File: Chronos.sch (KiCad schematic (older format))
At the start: 27 parts, among them Q1 NSS40301MZ4T1G, U1 ATMEGA32U2-AU, Y1 16MHz

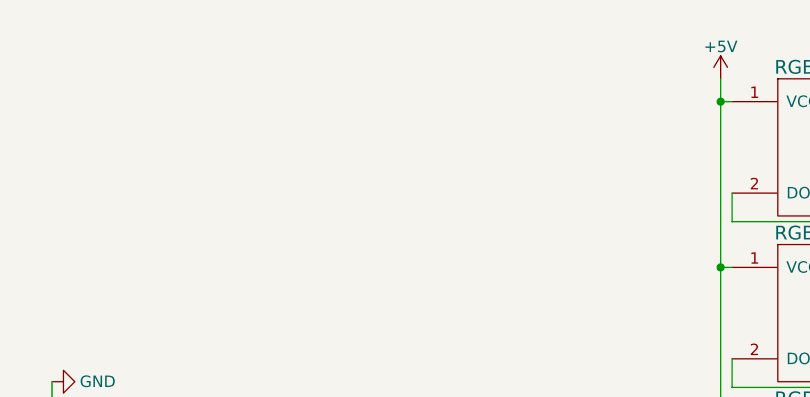
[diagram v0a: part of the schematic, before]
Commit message: Add RGB Decoupling capacitors
Also fix label on matrix sheet being misplaced
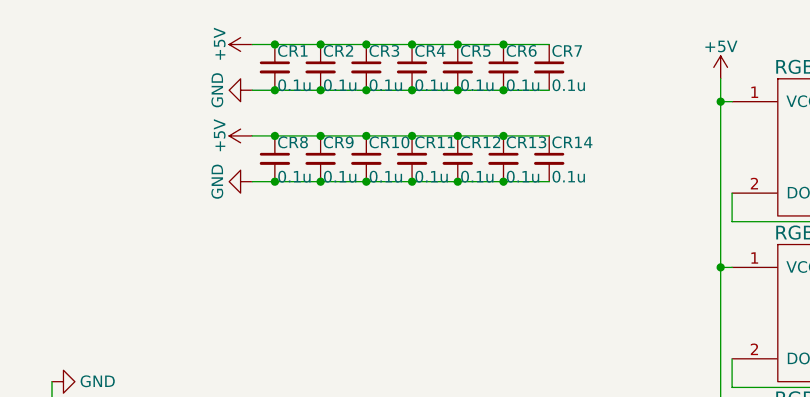
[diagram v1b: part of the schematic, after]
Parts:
- added CR1, CR10, CR11, CR12, CR13, CR14, CR2, CR3, CR4, CR5, CR6, CR7, CR8, CR9: 0.1u, symbol C_Small
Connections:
- net +5V: now also CR1.1, CR10.1, CR11.1, CR12.1, CR13.1, CR14.1, CR2.1, CR3.1, CR4.1, CR5.1, CR6.1, CR7.1, CR8.1, CR9.1
- net GND: now also CR1.2, CR10.2, CR11.2, CR12.2, CR13.2, CR14.2, CR2.2, CR3.2, CR4.2, CR5.2, CR6.2, CR7.2, CR8.2, CR9.2
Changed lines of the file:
@@
 Text Notes 8125 7650 0    60   ~ 0
 2017-10-15\n
+$Comp
+L C_Small CR1
+U 1 1 59E874F1
+P 6450 925
+F 0 "CR1" H 6460 995 50  0000 L CNN
+F 1 "0.1u" H 6460 845 50  0000 L CNN
+F 2 "" H 6450 925 50  0001 C CNN
+F 3 "" H 6450 925 50  0001 C CNN
+	1    6450 925
+	1    0    0    -1
+$EndComp
+$Comp
+L C_Small CR2
+U 1 1 59E879A6
+P 6650 925
+F 0 "CR2" H 6660 995 50  0000 L CNN
+F 1 "0.1u" H 6660 845 50  0000 L CNN
+F 2 "" H 6650 925 50  0001 C CNN
+F 3 "" H 6650 925 50  0001 C CNN
+	1    6650 925
+	1    0    0    -1
+$EndComp
+$Comp
+L C_Small CR3
+U 1 1 59E87A25
+P 6850 925
+F 0 "CR3" H 6860 995 50  0000 L CNN
+F 1 "0.1u" H 6860 845 50  0000 L CNN
+F 2 "" H 6850 925 50  0001 C CNN
+F 3 "" H 6850 925 50  0001 C CNN
+	1    6850 925
+	1    0    0    -1
+$EndComp
+$Comp
+L C_Small CR4
+U 1 1 59E87A9B
+P 7050 925
+F 0 "CR4" H 7060 995 50  0000 L CNN
+F 1 "0.1u" H 7060 845 50  0000 L CNN
+F 2 "" H 7050 925 50  0001 C CNN
+F 3 "" H 7050 925 50  0001 C CNN
+	1    7050 925
+	1    0    0    -1
+$EndComp
+$Comp
+L C_Small CR5
+U 1 1 59E87B14
+P 7250 925
+F 0 "CR5" H 7260 995 50  0000 L CNN
+F 1 "0.1u" H 7260 845 50  0000 L CNN
+F 2 "" H 7250 925 50  0001 C CNN
+F 3 "" H 7250 925 50  0001 C CNN
+	1    7250 925
+	1    0    0    -1
+$EndComp
+$Comp
+L C_Small CR6
+U 1 1 59E87B94
+P 7450 925
+F 0 "CR6" H 7460 995 50  0000 L CNN
+F 1 "0.1u" H 7460 845 50  0000 L CNN
+F 2 "" H 7450 925 50  0001 C CNN
+F 3 "" H 7450 925 50  0001 C CNN
+	1    7450 925
+	1    0    0    -1
+$EndComp
+$Comp
+L C_Small CR7
+U 1 1 59E87C1F
+P 7650 925
+F 0 "CR7" H 7660 995 50  0000 L CNN
+F 1 "0.1u" H 7660 845 50  0000 L CNN
+F 2 "" H 7650 925 50  0001 C CNN
+F 3 "" H 7650 925 50  0001 C CNN
+	1    7650 925
+	1    0    0    -1
+$EndComp
+Wire Wire Line
+	6350 825  7650 825
+Connection ~ 7450 825
+Connection ~ 7250 825
+Connection ~ 7050 825
+Connection ~ 6850 825
+Connection ~ 6650 825
+$Comp
+L +5V #PWR?
+U 1 1 59E88354
+P 6350 825
+F 0 "#PWR?" H 6350 675 50  0001 C CNN
+F 1 "+5V" H 6350 965 50  0000 C CNN
+F 2 "" H 6350 825 50  0001 C CNN
+F 3 "" H 6350 825 50  0001 C CNN
+	1    6350 825
+	0    -1   -1   0
+$EndComp
+Connection ~ 6450 825
+$Comp
+L GND #PWR?
+U 1 1 59E88464
+P 6350 1025
+F 0 "#PWR?" H 6350 775 50  0001 C CNN
+F 1 "GND" H 6350 875 50  0000 C CNN
+F 2 "" H 6350 1025 50  0001 C CNN
+F 3 "" H 6350 1025 50  0001 C CNN
+	1    6350 1025
+	0    1    1    0
+$EndComp
+Wire Wire Line
+	6350 1025 7650 1025
+Connection ~ 6450 1025
+Connection ~ 6650 1025
+Connection ~ 6850 1025
+Connection ~ 7050 1025
+Connection ~ 7250 1025
+Connection ~ 7450 1025
+$Comp
+L C_Small CR8
+U 1 1 59E89B67
+P 6450 1325
+F 0 "CR8" H 6460 1395 50  0000 L CNN
+F 1 "0.1u" H 6460 1245 50  0000 L CNN
+F 2 "" H 6450 1325 50  0001 C CNN
+F 3 "" H 6450 1325 50  0001 C CNN
+	1    6450 1325
+	1    0    0    -1
+$EndComp
+$Comp
+L C_Small CR9
+U 1 1 59E89B6D
+P 6650 1325
+F 0 "CR9" H 6660 1395 50  0000 L CNN
+F 1 "0.1u" H 6660 1245 50  0000 L CNN
+F 2 "" H 6650 1325 50  0001 C CNN
+F 3 "" H 6650 1325 50  0001 C CNN
+	1    6650 1325
+	1    0    0    -1
+$EndComp
+$Comp
+L C_Small CR10
+U 1 1 59E89B73
+P 6850 1325
+F 0 "CR10" H 6860 1395 50  0000 L CNN
+F 1 "0.1u" H 6860 1245 50  0000 L CNN
+F 2 "" H 6850 1325 50  0001 C CNN
+F 3 "" H 6850 1325 50  0001 C CNN
+	1    6850 1325
+	1    0    0    -1
+$EndComp
+$Comp
+L C_Small CR11
+U 1 1 59E89B79
+P 7050 1325
+F 0 "CR11" H 7060 1395 50  0000 L CNN
+F 1 "0.1u" H 7060 1245 50  0000 L CNN
+F 2 "" H 7050 1325 50  0001 C CNN
+F 3 "" H 7050 1325 50  0001 C CNN
+	1    7050 1325
+	1    0    0    -1
+$EndComp
+$Comp
+L C_Small CR12
+U 1 1 59E89B7F
+P 7250 1325
+F 0 "CR12" H 7260 1395 50  0000 L CNN
+F 1 "0.1u" H 7260 1245 50  0000 L CNN
+F 2 "" H 7250 1325 50  0001 C CNN
+F 3 "" H 7250 1325 50  0001 C CNN
+	1    7250 1325
+	1    0    0    -1
+$EndComp
+$Comp
+L C_Small CR13
+U 1 1 59E89B85
+P 7450 1325
+F 0 "CR13" H 7460 1395 50  0000 L CNN
+F 1 "0.1u" H 7460 1245 50  0000 L CNN
+F 2 "" H 7450 1325 50  0001 C CNN
+F 3 "" H 7450 1325 50  0001 C CNN
+	1    7450 1325
+	1    0    0    -1
+$EndComp
+$Comp
+L C_Small CR14
+U 1 1 59E89B8B
+P 7650 1325
+F 0 "CR14" H 7660 1395 50  0000 L CNN
+F 1 "0.1u" H 7660 1245 50  0000 L CNN
+F 2 "" H 7650 1325 50  0001 C CNN
+F 3 "" H 7650 1325 50  0001 C CNN
+	1    7650 1325
+	1    0    0    -1
+$EndComp
+Wire Wire Line
+	6350 1225 7650 1225
+Connection ~ 7450 1225
+Connection ~ 7250 1225
+Connection ~ 7050 1225
+Connection ~ 6850 1225
+Connection ~ 6650 1225
+$Comp
+L +5V #PWR?
+U 1 1 59E89B97
+P 6350 1225
+F 0 "#PWR?" H 6350 1075 50  0001 C CNN
+F 1 "+5V" H 6350 1365 50  0000 C CNN
+F 2 "" H 6350 1225 50  0001 C CNN
+F 3 "" H 6350 1225 50  0001 C CNN
+	1    6350 1225
+	0    -1   -1   0
+$EndComp
+Connection ~ 6450 1225
+$Comp
+L GND #PWR?
+U 1 1 59E89B9E
+P 6350 1425
+F 0 "#PWR?" H 6350 1175 50  0001 C CNN
+F 1 "GND" H 6350 1275 50  0000 C CNN
+F 2 "" H 6350 1425 50  0001 C CNN
+F 3 "" H 6350 1425 50  0001 C CNN
+	1    6350 1425
+	0    1    1    0
+$EndComp
+Wire Wire Line
+	6350 1425 7650 1425
+Connection ~ 6450 1425
+Connection ~ 6650 1425
+Connection ~ 6850 1425
+Connection ~ 7050 1425
+Connection ~ 7250 1425
+Connection ~ 7450 1425
 $EndSCHEMATC
